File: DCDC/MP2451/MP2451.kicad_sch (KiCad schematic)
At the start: 9 parts

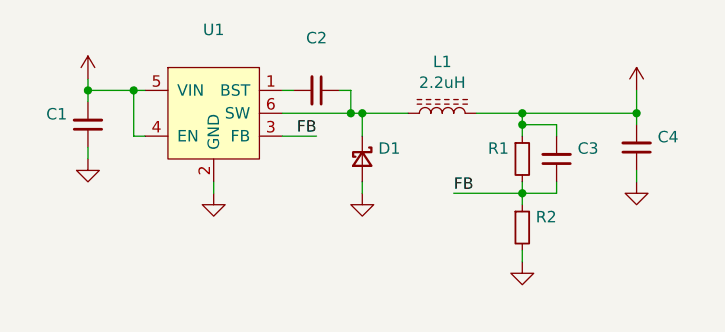
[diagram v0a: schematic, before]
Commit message: Reapply "Update modules to kicad v7 format"
This reverts commit fa5cc85431189ac7a3beedf0871b5723203ae43f.
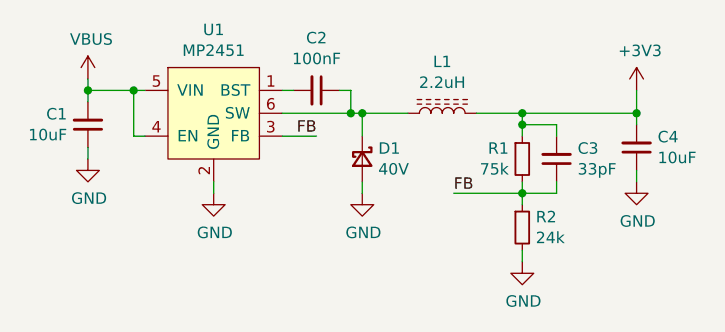
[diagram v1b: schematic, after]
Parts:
- C1: value (none) -> 10uF; footprint (none) -> Capacitor_SMD:C_1206_3216Metric
- C2: value (none) -> 100nF; footprint (none) -> Capacitor_SMD:C_0402_1005Metric
- C3: value (none) -> 33pF; footprint (none) -> Capacitor_SMD:C_0402_1005Metric
- C4: value (none) -> 10uF; footprint (none) -> Capacitor_SMD:C_0402_1005Metric
- D1: value (none) -> 40V; footprint (none) -> Diode_SMD:D_SOD-123
- R1: value (none) -> 75k; footprint (none) -> Resistor_SMD:R_0402_1005Metric
- R2: value (none) -> 24k; footprint (none) -> Resistor_SMD:R_0402_1005Metric
- U1: value (none) -> MP2451; footprint (none) -> Package_TO_SOT_SMD:SOT-23-6
